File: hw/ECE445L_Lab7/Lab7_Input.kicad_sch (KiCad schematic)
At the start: 2 parts

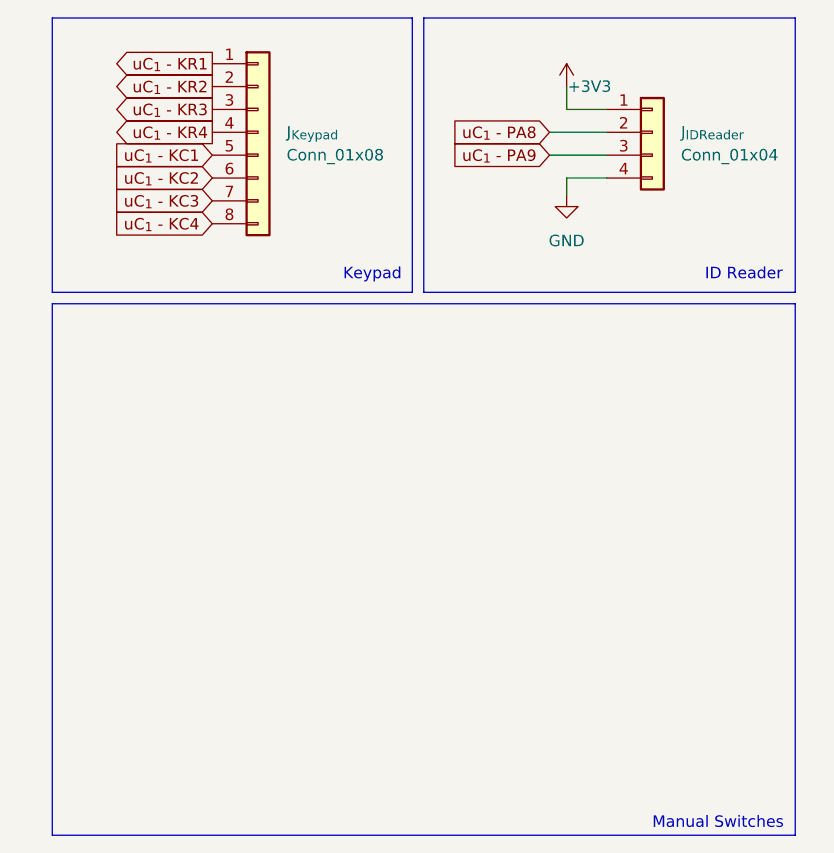
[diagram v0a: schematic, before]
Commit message: almost finished with schem
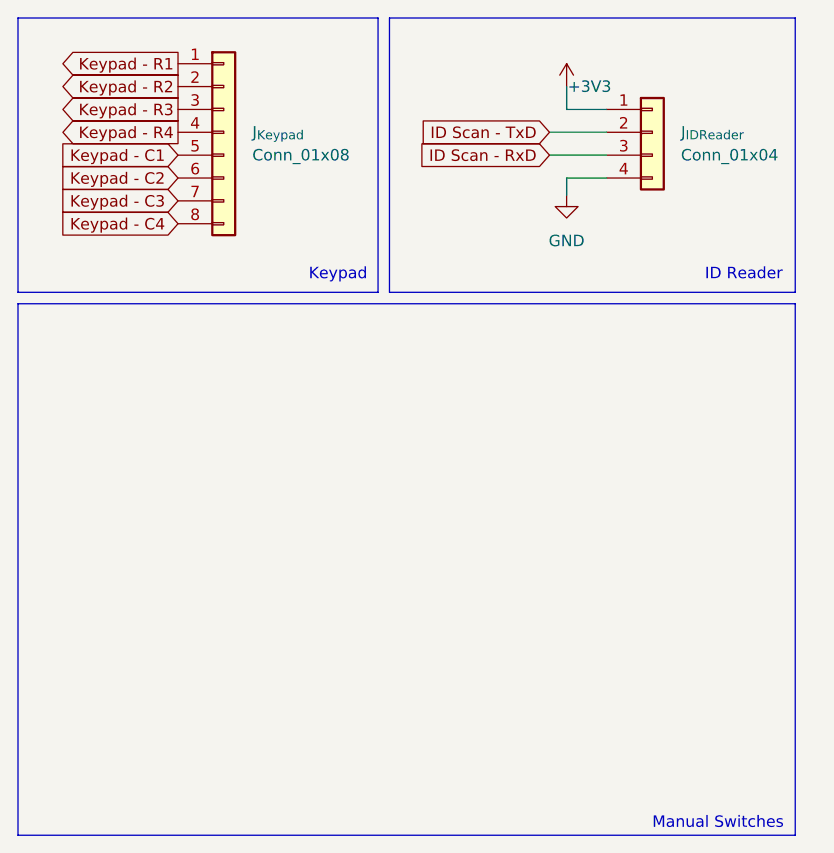
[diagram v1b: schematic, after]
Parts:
- J_{IDReader}: footprint (none) -> Connector_PinSocket_2.54mm:PinSocket_1x04_P2.54mm_Vertical
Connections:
- net uC_{1} - KC1 renamed Keypad - C1
- net uC_{1} - KC2 renamed Keypad - C2
- net uC_{1} - KC3 renamed Keypad - C3
- net uC_{1} - KC4 renamed Keypad - C4
- net uC_{1} - KR1 renamed Keypad - R1
- net uC_{1} - KR2 renamed Keypad - R2
- net uC_{1} - KR3 renamed Keypad - R3
- net uC_{1} - KR4 renamed Keypad - R4
- net uC_{1} - PA8 renamed ID Scan - TxD
- net uC_{1} - PA9 renamed ID Scan - RxD
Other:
- moved on the sheet: J_{Keypad}
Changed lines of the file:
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@@
 	)
 	(rectangle
-		(start 69.85 34.925)
-		(end 109.855 65.405)
+		(start 66.04 34.925)
+		(end 106.045 65.405)
 		(stroke
 			(width 0)
@@
 	)
 	(rectangle
-		(start 111.125 34.925)
+		(start 107.315 34.925)
 		(end 152.4 65.405)
 		(stroke
@@
 	)
 	(rectangle
-		(start 69.85 66.675)
+		(start 66.04 66.675)
 		(end 152.4 125.73)
 		(stroke
@@
 	(text "Keypad"
 		(exclude_from_sim no)
-		(at 105.41 63.5 0)
+		(at 101.6 63.5 0)
 		(effects
 			(font
@@
 		)
 	)
-	(global_label "uC_{1} - KR1"
+	(global_label "Keypad - R1"
 		(shape output)
-		(at 87.63 40.005 180)
-		(fields_autoplaced yes)
-		(effects
-			(font
-				(size 1.27 1.27)
-			)
-			(justify right)
-		)
-		(property "Intersheetrefs" "${INTERSHEET_REFS}"
-			(at 74.0011 40.005 0)
-			(hide yes)
-			(show_name no)
-			(do_not_autoplace no)
-			(effects
-				(font
-					(size 1.27 1.27)
-				)
-				(justify right)
-			)
-		)
-	)
-	(global_label "uC_{1} - PA8"
+		(at 83.82 40.005 180)
+		(fields_autoplaced yes)
+		(effects
+			(font
+				(size 1.27 1.27)
+			)
+			(justify right)
+		)
+		(property "Intersheetrefs" "${INTERSHEET_REFS}"
+			(at 70.1911 40.005 0)
+			(hide yes)
+			(show_name no)
+			(do_not_autoplace no)
+			(effects
+				(font
+					(size 1.27 1.27)
+				)
+				(justify right)
+			)
+		)
+	)
+	(global_label "ID Scan - TxD"
 		(shape input)
 		(at 125.095 47.625 180)
@@
 		)
 	)
-	(global_label "uC_{1} - KR3"
+	(global_label "Keypad - R3"
 		(shape output)
-		(at 87.63 45.085 180)
-		(fields_autoplaced yes)
-		(effects
-			(font
-				(size 1.27 1.27)
-			)
-			(justify right)
-		)
-		(property "Intersheetrefs" "${INTERSHEET_REFS}"
-			(at 74.0011 45.085 0)
-			(hide yes)
-			(show_name no)
-			(do_not_autoplace no)
-			(effects
-				(font
-					(size 1.27 1.27)
-				)
-				(justify right)
-			)
-		)
-	)
-	(global_label "uC_{1} - KC4"
+		(at 83.82 45.085 180)
+		(fields_autoplaced yes)
+		(effects
+			(font
+				(size 1.27 1.27)
+			)
+			(justify right)
+		)
+		(property "Intersheetrefs" "${INTERSHEET_REFS}"
+			(at 70.1911 45.085 0)
+			(hide yes)
+			(show_name no)
+			(do_not_autoplace no)
+			(effects
+				(font
+					(size 1.27 1.27)
+				)
+				(justify right)
+			)
+		)
+	)
+	(global_label "Keypad - C4"
 		(shape input)
-		(at 87.63 57.785 180)
-		(fields_autoplaced yes)
-		(effects
-			(font
-				(size 1.27 1.27)
-			)
-			(justify right)
-		)
-		(property "Intersheetrefs" "${INTERSHEET_REFS}"
-			(at 74.0011 57.785 0)
-			(hide yes)
-			(show_name no)
-			(do_not_autoplace no)
-			(effects
-				(font
-					(size 1.27 1.27)
-				)
-				(justify right)
-			)
-		)
-	)
-	(global_label "uC_{1} - KC2"
+		(at 83.82 57.785 180)
+		(fields_autoplaced yes)
+		(effects
+			(font
+				(size 1.27 1.27)
+			)
+			(justify right)
+		)
+		(property "Intersheetrefs" "${INTERSHEET_REFS}"
+			(at 70.1911 57.785 0)
+			(hide yes)
+			(show_name no)
+			(do_not_autoplace no)
+			(effects
+				(font
+					(size 1.27 1.27)
+				)
+				(justify right)
+			)
+		)
+	)
+	(global_label "Keypad - C2"
 		(shape input)
-		(at 87.63 52.705 180)
-		(fields_autoplaced yes)
-		(effects
-			(font
-				(size 1.27 1.27)
-			)
-			(justify right)
-		)
-		(property "Intersheetrefs" "${INTERSHEET_REFS}"
-			(at 74.0011 52.705 0)
-			(hide yes)
-			(show_name no)
-			(do_not_autoplace no)
-			(effects
-				(font
-					(size 1.27 1.27)
-				)
-				(justify right)
-			)
-		)
-	)
-	(global_label "uC_{1} - KR2"
+		(at 83.82 52.705 180)
+		(fields_autoplaced yes)
+		(effects
+			(font
+				(size 1.27 1.27)
+			)
+			(justify right)
+		)
+		(property "Intersheetrefs" "${INTERSHEET_REFS}"
+			(at 70.1911 52.705 0)
+			(hide yes)
+			(show_name no)
+			(do_not_autoplace no)
+			(effects
+				(font
+					(size 1.27 1.27)
+				)
+				(justify right)
+			)
+		)
+	)
+	(global_label "Keypad - R2"
 		(shape output)
-		(at 87.63 42.545 180)
-		(fields_autoplaced yes)
-		(effects
-			(font
-				(size 1.27 1.27)
-			)
-			(justify right)
-		)
-		(property "Intersheetrefs" "${INTERSHEET_REFS}"
-			(at 74.0011 42.545 0)
-			(hide yes)
-			(show_name no)
-			(do_not_autoplace no)
-			(effects
-				(font
-					(size 1.27 1.27)
-				)
-				(justify right)
-			)
-		)
-	)
-	(global_label "uC_{1} - KC1"
+		(at 83.82 42.545 180)
+		(fields_autoplaced yes)
+		(effects
+			(font
+				(size 1.27 1.27)
+			)
+			(justify right)
+		)
+		(property "Intersheetrefs" "${INTERSHEET_REFS}"
+			(at 70.1911 42.545 0)
+			(hide yes)
+			(show_name no)
+			(do_not_autoplace no)
+			(effects
+				(font
+					(size 1.27 1.27)
+				)
+				(justify right)
+			)
+		)
+	)
+	(global_label "Keypad - C1"
 		(shape input)
-		(at 87.63 50.165 180)
-		(fields_autoplaced yes)
-		(effects
-			(font
-				(size 1.27 1.27)
-			)
-			(justify right)
-		)
-		(property "Intersheetrefs" "${INTERSHEET_REFS}"
-			(at 74.0011 50.165 0)
-			(hide yes)
-			(show_name no)
-			(do_not_autoplace no)
-			(effects
-				(font
-					(size 1.27 1.27)
-				)
-				(justify right)
-			)
-		)
-	)
-	(global_label "uC_{1} - PA9"
+		(at 83.82 50.165 180)
+		(fields_autoplaced yes)
+		(effects
+			(font
+				(size 1.27 1.27)
+			)
+			(justify right)
+		)
+		(property "Intersheetrefs" "${INTERSHEET_REFS}"
+			(at 70.1911 50.165 0)
+			(hide yes)
+			(show_name no)
+			(do_not_autoplace no)
+			(effects
+				(font
+					(size 1.27 1.27)
+				)
+				(justify right)
+			)
+		)
+	)
+	(global_label "ID Scan - RxD"
 		(shape input)
 		(at 125.095 50.165 180)
@@
 		)
 	)
-	(global_label "uC_{1} - KC3"
+	(global_label "Keypad - C3"
 		(shape input)
-		(at 87.63 55.245 180)
-		(fields_autoplaced yes)
-		(effects
-			(font
-				(size 1.27 1.27)
-			)
-			(justify right)
-		)
-		(property "Intersheetrefs" "${INTERSHEET_REFS}"
-			(at 74.0011 55.245 0)
-			(hide yes)
-			(show_name no)
-			(do_not_autoplace no)
-			(effects
-				(font
-					(size 1.27 1.27)
-				)
-				(justify right)
-			)
-		)
-	)
-	(global_label "uC_{1} - KR4"
+		(at 83.82 55.245 180)
+		(fields_autoplaced yes)
+		(effects
+			(font
+				(size 1.27 1.27)
+			)
+			(justify right)
+		)
+		(property "Intersheetrefs" "${INTERSHEET_REFS}"
+			(at 70.1911 55.245 0)
+			(hide yes)
+			(show_name no)
+			(do_not_autoplace no)
+			(effects
+				(font
+					(size 1.27 1.27)
+				)
+				(justify right)
+			)
+		)
+	)
+	(global_label "Keypad - R4"
 		(shape output)
-		(at 87.63 47.625 180)
-		(fields_autoplaced yes)
-		(effects
-			(font
-				(size 1.27 1.27)
-			)
-			(justify right)
-		)
-		(property "Intersheetrefs" "${INTERSHEET_REFS}"
-			(at 74.0011 47.625 0)
+		(at 83.82 47.625 180)
+		(fields_autoplaced yes)
+		(effects
+			(font
+				(size 1.27 1.27)
+			)
+			(justify right)
+		)
+		(property "Intersheetrefs" "${INTERSHEET_REFS}"
+			(at 70.1911 47.625 0)
 			(hide yes)
 			(show_name no)
@@
 	(symbol
 		(lib_id "Connector_Generic:Conn_01x08")
-		(at 92.71 47.625 0)
+		(at 88.9 47.625 0)
 		(unit 1)
 		(body_style 1)
@@
 		(fields_autoplaced yes)
 		(property "Reference" "J_{Keypad}"
-			(at 95.885 47.6249 0)
+			(at 92.075 47.6249 0)
 			(show_name no)
 			(do_not_autoplace no)
@@
 		)
 		(property "Value" "Conn_01x08"
-			(at 95.885 50.1649 0)
+			(at 92.075 50.1649 0)
 			(show_name no)
 			(do_not_autoplace no)
@@
 		)
 		(property "Footprint" "Connector_PinSocket_2.54mm:PinSocket_1x08_P2.54mm_Vertical"
-			(at 92.71 47.625 0)
+			(at 88.9 47.625 0)
 			(hide yes)
 			(show_name no)
@@
 		)
 		(property "Datasheet" ""
-			(at 92.71 47.625 0)
+			(at 88.9 47.625 0)
 			(hide yes)
 			(show_name no)
@@
 		)
 		(property "Description" "Generic connector, single row, 01x08, script generated (kicad-library-utils/schlib/autogen/connector/)"
-			(at 92.71 47.625 0)
+			(at 88.9 47.625 0)
 			(hide yes)
 			(show_name no)
@@
 			)
 		)
-		(property "Footprint" ""
+		(property "Footprint" "Connector_PinSocket_2.54mm:PinSocket_1x04_P2.54mm_Vertical"
 			(at 136.525 47.625 0)
 			(hide yes)

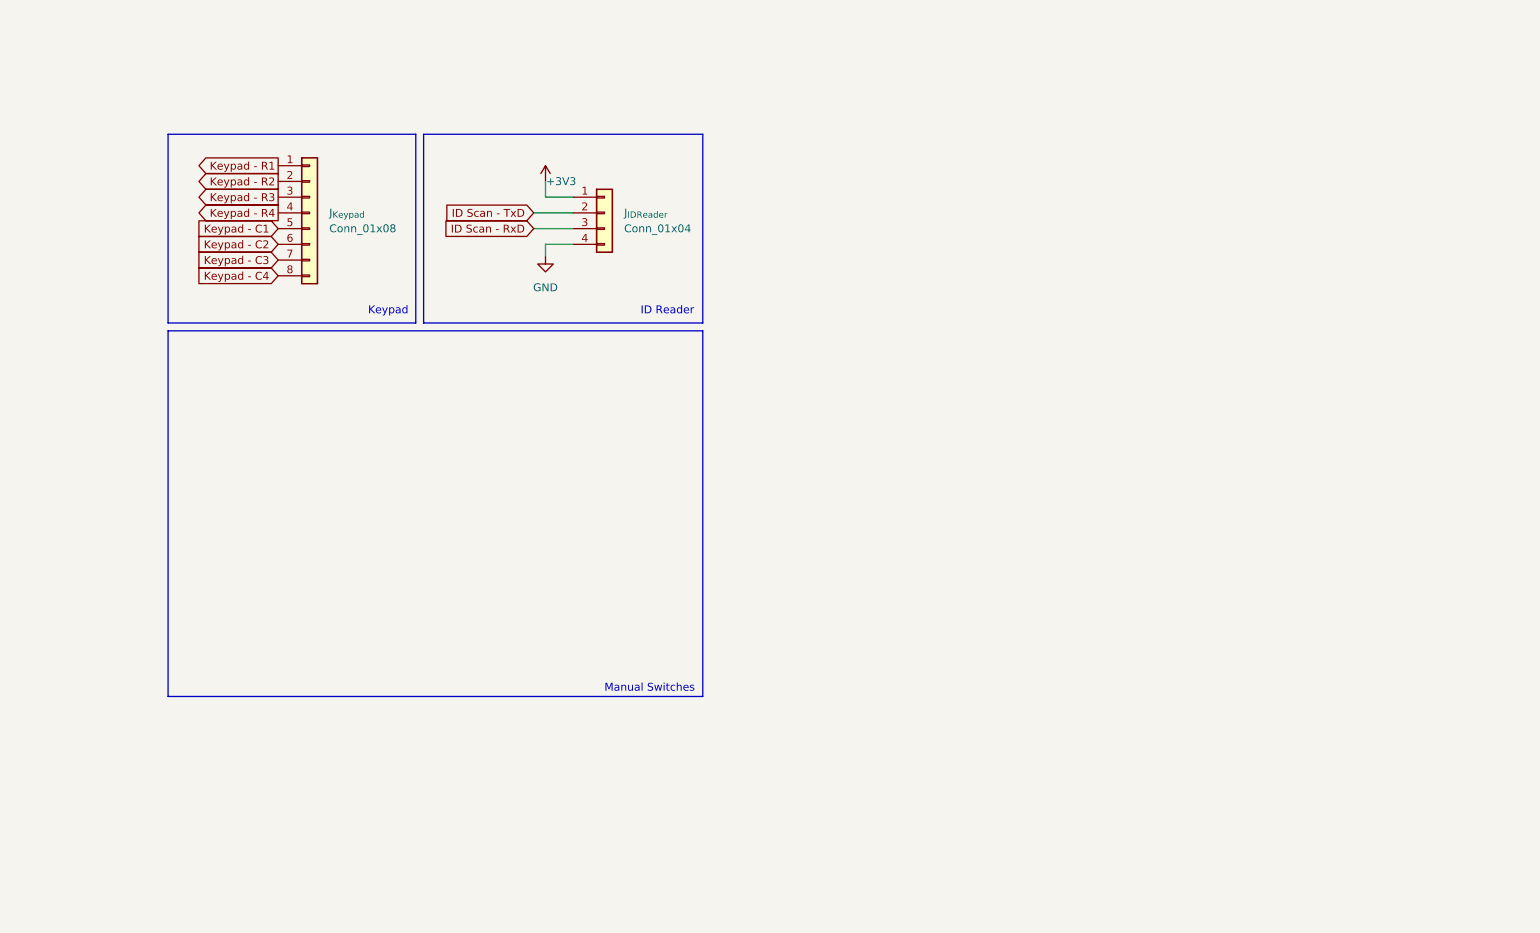
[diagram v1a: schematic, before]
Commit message: finished prelim schem
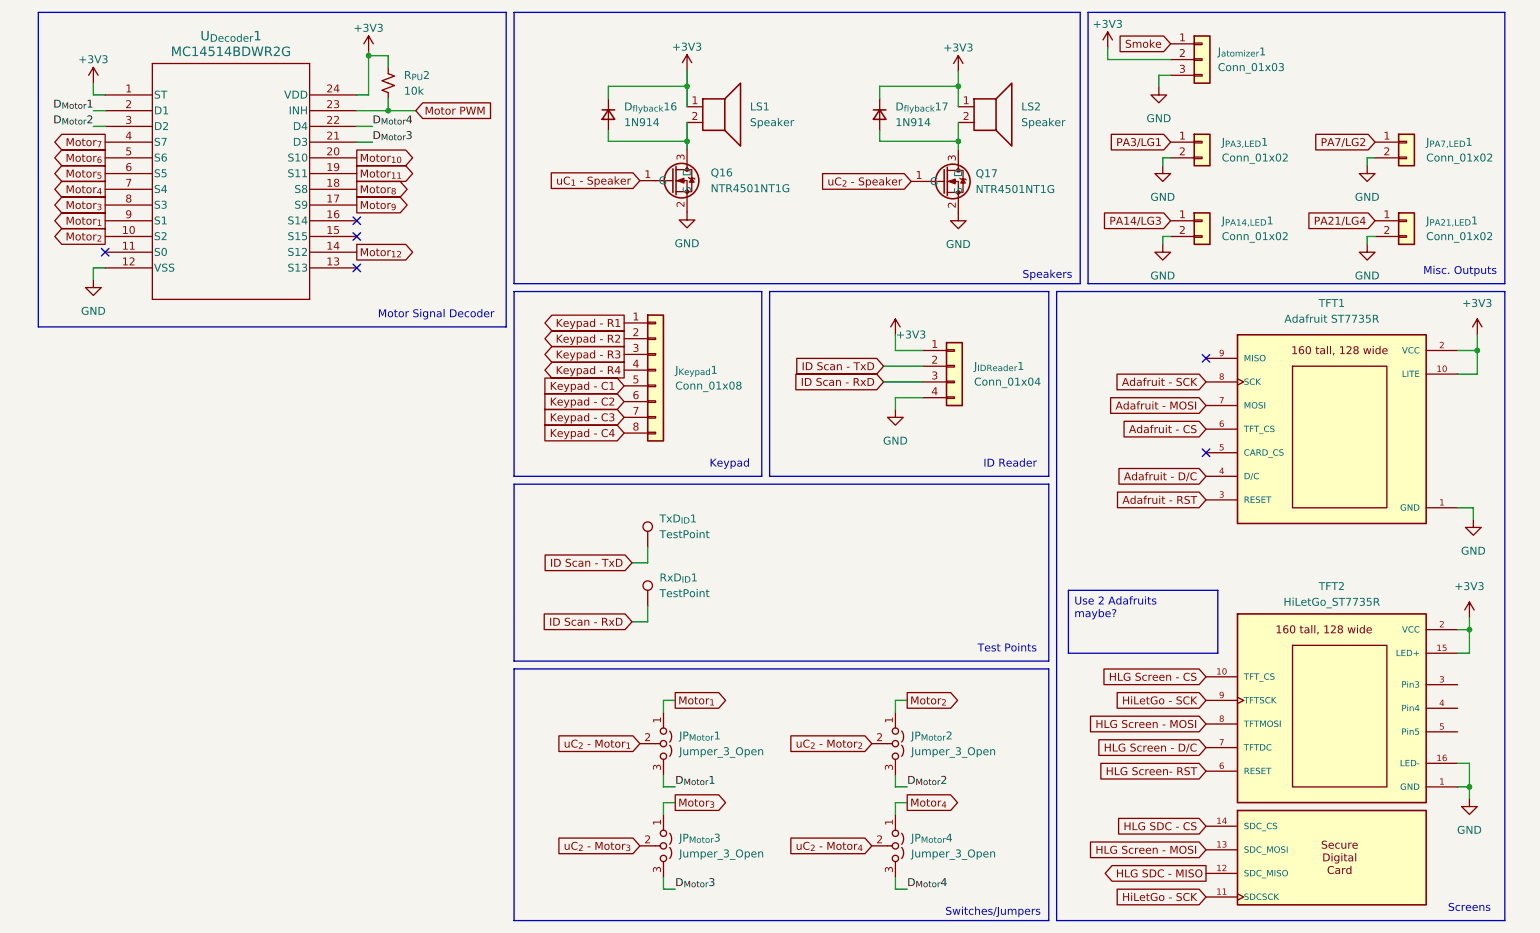
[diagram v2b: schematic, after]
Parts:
- added D_{flyback}16, D_{flyback}17: 1N914, Diode_THT:D_5W_P12.70mm_Horizontal, symbol Device:D_Small
- added JP_{Motor}1, JP_{Motor}2, JP_{Motor}3, JP_{Motor}4: Jumper_3_Open, Connector_PinHeader_2.54mm:PinHeader_1x03_P2.54mm_Vertical, symbol Jumper:Jumper_3_Open
- added J_{PA14,LED}1, J_{PA21,LED}1, J_{PA3,LED}1, J_{PA7,LED}1: Conn_01x02, Connector_PinSocket_2.54mm:PinSocket_1x02_P2.54mm_Vertical, symbol Connector_Generic:Conn_01x02
- added J_{atomizer}1: Conn_01x03, Connector_PinSocket_2.54mm:PinSocket_1x03_P2.54mm_Vertical, symbol Connector_Generic:Conn_01x03
- added LS1, LS2: Speaker, ECE445L:PinHeader_1x02_P2.54mm_Vertical, symbol ECE445L:Speaker
- added Q16, Q17: NTR4501NT1G, ECE445L:SOT96P237X111-3N, symbol ECE445L:NTR4501NT1G
- added R_{PU}2: 10k, Resistor_SMD:R_0805_2012Metric_Pad1.20x1.40mm_HandSolder, symbol ECE445L:R_0.125W
- added RxD_{ID}1, TxD_{ID}1: TestPoint, TestPoint:TestPoint_Keystone_5010-5014_Multipurpose, symbol Connector:TestPoint
- added TFT1: Adafruit ST7735R, ECE445L:adafruit_st7735r2, symbol ECE445L:Adafruit_ST7735R
- added TFT2: HiLetGo_ST7735R, ECE445L:hiletgo_st7735r2, symbol ECE445L:HiLetGo_ST7735R
- added U_{Decoder}1: MC14514BDWR2G, ECE445L:SOIC-24WB_ONS, symbol ECE445L:MC14514BDWR2G
- J_{Keypad}1: renamed from J_{Keypad}; footprint Connector_PinSocket_2.54mm:PinSocket_1x08_P2.54mm_Vertical -> ECE445L:4x4_Matrix_Keypad
- renumbered J_{IDReader} to J_{IDReader}1
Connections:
- net +3V3: now also D_{flyback}16.1 (K), D_{flyback}17.1 (K), J_{atomizer}1.2 (Pin_2), LS1.1, LS2.1, R_{PU}2.1, TFT1.10 (LITE), TFT1.2 (VCC), TFT2.15 (LED+), TFT2.2 (VCC), U_{Decoder}1.1 (ST), U_{Decoder}1.24 (VDD)
- net GND: now also J_{PA14,LED}1.2 (Pin_2), J_{PA21,LED}1.2 (Pin_2), J_{PA3,LED}1.2 (Pin_2), J_{PA7,LED}1.2 (Pin_2), J_{atomizer}1.3 (Pin_3), Q16.2 (S), Q17.2 (S), TFT1.1 (GND), TFT2.1 (GND), TFT2.16 (LED-), U_{Decoder}1.12 (VSS)
- net ID Scan - RxD: now also RxD_{ID}1.1
- net ID Scan - TxD: now also TxD_{ID}1.1
- new net: D_{flyback}17.2 (A), LS2.2, Q17.3 (D)
- new net: D_{flyback}16.2 (A), LS1.2, Q16.3 (D)
- new net Adafruit - CS: TFT1.6 (TFT_CS)
- new net Adafruit - D/C: TFT1.4 (D/C)
- new net Adafruit - MOSI: TFT1.7 (MOSI)
- new net Adafruit - RST: TFT1.3 (RESET)
- new net Adafruit - SCK: TFT1.8 (SCK)
- new net D_{Motor}1: JP_{Motor}1.3 (B), U_{Decoder}1.2 (D1)
- new net D_{Motor}2: JP_{Motor}2.3 (B), U_{Decoder}1.3 (D2)
- new net D_{Motor}3: JP_{Motor}3.3 (B), U_{Decoder}1.21 (D3)
- new net D_{Motor}4: JP_{Motor}4.3 (B), U_{Decoder}1.22 (D4)
- new net HLG SDC - CS: TFT2.14 (SDC_CS)
- new net HLG SDC - MISO: TFT2.12 (SDC_MISO)
- new net HLG Screen - CS: TFT2.10 (TFT_CS)
- new net HLG Screen - D/C: TFT2.7 (TFTDC)
- new net HLG Screen - MOSI: TFT2.13 (SDC_MOSI), TFT2.8 (TFTMOSI)
- new net HLG Screen- RST: TFT2.6 (RESET)
- new net HiLetGo - SCK: TFT2.11 (SDCSCK), TFT2.9 (TFTSCK)
- new net Motor PWM: R_{PU}2.2, U_{Decoder}1.23 (INH)
- new net Motor_{10}: U_{Decoder}1.20 (S10)
- new net Motor_{11}: U_{Decoder}1.19 (S11)
- new net Motor_{12}: U_{Decoder}1.14 (S12)
- new net Motor_{1}: JP_{Motor}1.1 (A), U_{Decoder}1.9 (S1)
- new net Motor_{2}: JP_{Motor}2.1 (A), U_{Decoder}1.10 (S2)
- new net Motor_{3}: JP_{Motor}3.1 (A), U_{Decoder}1.8 (S3)
- new net Motor_{4}: JP_{Motor}4.1 (A), U_{Decoder}1.7 (S4)
- new net Motor_{5}: U_{Decoder}1.6 (S5)
- new net Motor_{6}: U_{Decoder}1.5 (S6)
- new net Motor_{7}: U_{Decoder}1.4 (S7)
- new net Motor_{8}: U_{Decoder}1.18 (S8)
- new net Motor_{9}: U_{Decoder}1.17 (S9)
- new net PA14/LG3: J_{PA14,LED}1.1 (Pin_1)
- new net PA21/LG4: J_{PA21,LED}1.1 (Pin_1)
- new net PA3/LG1: J_{PA3,LED}1.1 (Pin_1)
- new net PA7/LG2: J_{PA7,LED}1.1 (Pin_1)
- new net Smoke: J_{atomizer}1.1 (Pin_1)
- new net uC_{1} - Speaker: Q16.1 (G)
- new net uC_{2} - Motor_{1}: JP_{Motor}1.2 (C)
- new net uC_{2} - Motor_{2}: JP_{Motor}2.2 (C)
- new net uC_{2} - Motor_{3}: JP_{Motor}3.2 (C)
- new net uC_{2} - Motor_{4}: JP_{Motor}4.2 (C)
- new net uC_{2} - Speaker: Q17.1 (G)
- no-connect marks 0 -> 6
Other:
- note added: "Misc. Outputs"
- note added: "Motor Signal Decoder"
- note added: "Screens"
- note added: "Speakers"
- note added: "Switches/Jumpers"
- note added: "Test Points"
- note removed: "Manual Switches"
- moved on the sheet: J_{IDReader}1, J_{Keypad}1
